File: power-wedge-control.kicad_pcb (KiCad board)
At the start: 2 copper layers, 77.2 x 64.5 mm, 89 parts, among them J1 Conn_01x02, J10 Conn_01x10, J11 Conn_01x08, J12 Conn_01x06, J2 Conn_01x03, J3 Conn_01x02, J4 Conn_01x03, J5 Conn_01x03, J6 Conn_01x06_Female, J7 Conn_01x04_Female, J8 Conn_01x04, J9 MicroSD_Hirose_DM3D-SF, Q1 MMBT3904L, Q2 DMP3099L, Q3 MMBT3904L, Q4 DMP3099L, Q5 MMBT3904L, Q6 MMBT3904L, SW1 SW_SPST, U1 LM1117-5.0, U10 74LVC1G32, U11 74LVC1G32, U2 NC7WZ14P6X, U3 TLV70233DBV, U4 LTV-817S, U5 NC7WZ17P6X, U6 NC7WZ17P6X, U7 LTV-817S, U8 SN74LVC08ADRG3, U9 NC7WZ14P6X

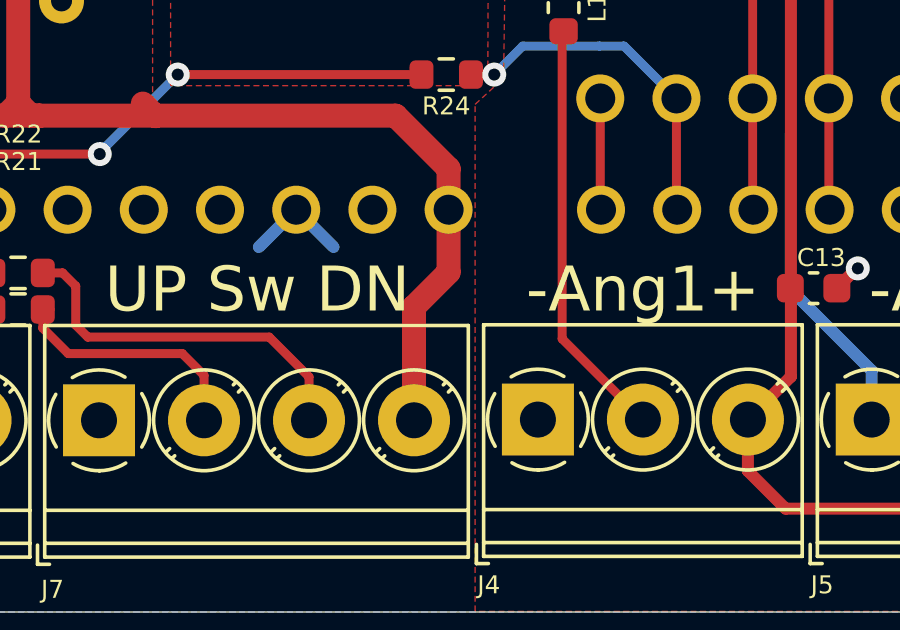
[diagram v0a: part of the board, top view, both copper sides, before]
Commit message: Add 470 Ω resistor to limit current on +12V pin to up/down buttons.
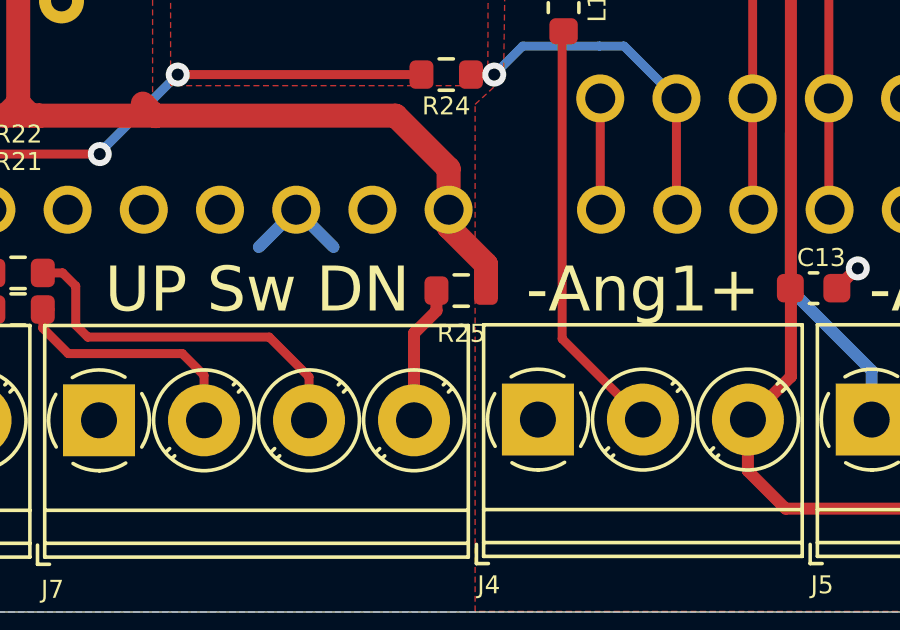
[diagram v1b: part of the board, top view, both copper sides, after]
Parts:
- added R25: 470, Resistor_SMD:R_0603_1608Metric, F.Cu at (168.2, 130.3)
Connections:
- J7 pad 4: +12V -> Net-(J7-Pad4)
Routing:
- net Net-(J7-Pad4): track 0.00 -> 4.63 mm
- net +12V: track 96.6 -> 92.3 mm
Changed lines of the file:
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@@
   (net 80 "Net-(U10-Pad1)")
   (net 81 "Net-(U11-Pad1)")
+  (net 82 "Net-(J7-Pad4)")
   (footprint "TerminalBlock_Phoenix:TerminalBlock_Phoenix_PT-1,5-2-3.5-H_1x02_P3.50mm_Horizontal" (layer "F.Cu")
     (at 126.9088 134.6554)
@@
     )
   )
+  (footprint "Resistor_SMD:R_0603_1608Metric" (layer "F.Cu")
+    (at 168.188 130.331 180)
+    (descr "Resistor SMD 0603 (1608 Metric), square (rectangular) end terminal, IPC_7351 nominal, (Body size source: IPC-SM-782 page 72, https://www.pcb-3d.com/wordpress/wp-content/uploads/ipc-sm-782a_amendment_1_and_2.pdf), generated with kicad-footprint-generator")
+    (tags "resistor")
+    (property "Sheetfile" "power-wedge-control.kicad_sch")
+    (property "Sheetname" "")
+    (attr smd)
+    (fp_text reference "R25" (at 0 -1.43) (layer "F.SilkS")
+      (effects (font (size 0.6 0.6) (thickness 0.15)))
+    )
+    (fp_text value "470" (at 0 1.43) (layer "F.Fab")
+      (effects (font (size 1 1) (thickness 0.15)))
+    )
+    (fp_text user "${REFERENCE}" (at 0 0) (layer "F.Fab")
+      (effects (font (size 0.6 0.6) (thickness 0.06)))
+    )
+    (fp_line (start -0.237258 0.5225) (end 0.237258 0.5225) (layer "F.SilkS") (width 0.12))
+    (fp_line (start -0.237258 -0.5225) (end 0.237258 -0.5225) (layer "F.SilkS") (width 0.12))
+    (fp_line (start -1.48 0.73) (end -1.48 -0.73) (layer "F.CrtYd") (width 0.05))
+    (fp_line (start -1.48 -0.73) (end 1.48 -0.73) (layer "F.CrtYd") (width 0.05))
+    (fp_line (start 1.48 -0.73) (end 1.48 0.73) (layer "F.CrtYd") (width 0.05))
+    (fp_line (start 1.48 0.73) (end -1.48 0.73) (layer "F.CrtYd") (width 0.05))
+    (fp_line (start 0.8 -0.4125) (end 0.8 0.4125) (layer "F.Fab") (width 0.1))
+    (fp_line (start -0.8 0.4125) (end -0.8 -0.4125) (layer "F.Fab") (width 0.1))
+    (fp_line (start -0.8 -0.4125) (end 0.8 -0.4125) (layer "F.Fab") (width 0.1))
+    (fp_line (start 0.8 0.4125) (end -0.8 0.4125) (layer "F.Fab") (width 0.1))
+    (pad "1" smd roundrect (at -0.825 0 180) (size 0.8 0.95) (layers "F.Cu" "F.Paste" "F.Mask") (roundrect_rratio 0.25)
+      (net 4 "+12V") (pintype "passive"))
+    (pad "2" smd roundrect (at 0.825 0 180) (size 0.8 0.95) (layers "F.Cu" "F.Paste" "F.Mask") (roundrect_rratio 0.25)
+      (net 82 "Net-(J7-Pad4)") (pintype "passive"))
+    (model "${KICAD6_3DMODEL_DIR}/Resistor_SMD.3dshapes/R_0603_1608Metric.wrl"
+      (offset (xyz 0 0 0))
+      (scale (xyz 1 1 1))
+      (rotate (xyz 0 0 0))
+    )
+  )
   (footprint "Capacitor_SMD:C_0603_1608Metric" (layer "F.Cu")
     (at 179.9336 130.2512)
@@
       (net 70 "/SW2EXT") (pinfunction "Pin_3") (pintype "passive"))
     (pad "4" thru_hole circle locked (at 10.5 0) (size 2.4 2.4) (drill 1.2) (layers *.Cu *.Mask)
-      (net 4 "+12V") (pinfunction "Pin_4") (pintype "passive"))
+      (net 82 "Net-(J7-Pad4)") (pinfunction "Pin_4") (pintype "passive"))
     (model "${KICAD6_3DMODEL_DIR}/TerminalBlock_Phoenix.3dshapes/TerminalBlock_Phoenix_PT-1,5-4-3.5-H_1x04_P3.50mm_Horizontal.wrl"
       (offset (xyz 0 0 0))
@@
   (segment (start 115.8224 124.8664) (end 115.8224 123.4668) (width 0.8) (layer "F.Cu") (net 3))
   (segment (start 153 124.5) (end 154.138 124.5) (width 0.8) (layer "F.Cu") (net 4))
+  (segment (start 169.013 130.331) (end 169.013 129.456) (width 0.8) (layer "F.Cu") (net 4))
   (segment (start 154.9562 115.9502) (end 155.6562 115.2502) (width 0.8) (layer "F.Cu") (net 4))
   (segment (start 119.198 120.4346) (end 119.198 119.0244) (width 0.8) (layer "F.Cu") (net 4))
@@
   (segment (start 154.138 124.5) (end 166 124.5) (width 0.8) (layer "F.Cu") (net 4))
   (segment (start 153.421 115.9502) (end 153.421 124.079) (width 0.8) (layer "F.Cu") (net 4))
-  (segment (start 167.767 129.7178) (end 166.6136 130.8712) (width 0.8) (layer "F.Cu") (net 4))
   (segment (start 127.741518 124.499118) (end 126.9088 125.331836) (width 0.8) (layer "F.Cu") (net 4))
   (segment (start 154.138 124.5) (end 153.842 124.5) (width 0.8) (layer "F.Cu") (net 4))
-  (segment (start 166.6136 130.8712) (end 166.6136 134.6554) (width 0.8) (layer "F.Cu") (net 4))
   (segment (start 126.119 120.4346) (end 126.6656 119.888) (width 0.8) (layer "F.Cu") (net 4))
   (segment (start 132.650482 124.499118) (end 132.6878 124.4618) (width 0.8) (layer "F.Cu") (net 4))
@@
   (segment (start 122.566 119.0092) (end 122.6524 118.9228) (width 0.8) (layer "F.Cu") (net 4))
   (segment (start 126.9088 125.331836) (end 126.9088 134.6554) (width 0.8) (layer "F.Cu") (net 4))
-  (segment (start 167.767 127.635) (end 167.767 129.7178) (width 0.8) (layer "F.Cu") (net 4))
   (segment (start 147.8788 124.5) (end 153 124.5) (width 0.8) (layer "F.Cu") (net 4))
   (segment (start 126.056 120.4346) (end 126.119 120.4346) (width 0.8) (layer "F.Cu") (net 4))
@@
   (segment (start 155.6562 115.2502) (end 155.6562 116.3832) (width 0.8) (layer "F.Cu") (net 4))
   (segment (start 116.5056 118.9228) (end 119.0964 118.9228) (width 0.8) (layer "F.Cu") (net 4))
+  (segment (start 169.013 129.456) (end 167.767 128.21) (width 0.8) (layer "F.Cu") (net 4))
   (segment (start 115.708 120.7562) (end 115.708 119.7204) (width 0.8) (layer "F.Cu") (net 4))
   (segment (start 125.7004 118.9228) (end 126.6656 119.888) (width 0.8) (layer "F.Cu") (net 4))
   (segment (start 153.842 124.5) (end 153.421 124.079) (width 0.8) (layer "F.Cu") (net 4))
   (segment (start 153.421 124.079) (end 153 124.5) (width 0.8) (layer "F.Cu") (net 4))
+  (segment (start 167.767 128.21) (end 167.767 127.635) (width 0.8) (layer "F.Cu") (net 4))
   (segment (start 142.388 124.481) (end 132.650482 124.499118) (width 0.8) (layer "F.Cu") (net 4))
   (via (at 147.8788 124.5) (size 1.6) (drill 0.8) (layers "F.Cu" "B.Cu") (net 4))
@@
   (segment (start 128.239519 94.874519) (end 128.89 95.525) (width 0.3) (layer "F.Cu") (net 81))
   (segment (start 128.89 95.525) (end 128.89 97.7) (width 0.3) (layer "F.Cu") (net 81))
+  (segment (start 167.363 130.331) (end 167.363 131.006) (width 0.4) (layer "F.Cu") (net 82))
+  (segment (start 167.363 131.006) (end 166.6136 131.7554) (width 0.4) (layer "F.Cu") (net 82))
+  (segment (start 166.6136 131.7554) (end 166.6136 134.6554) (width 0.4) (layer "F.Cu") (net 82))
   (zone (net 0) (net_name "") (layer "F.Cu") (hatch edge 0.508)
     (connect_pads (clearance 0))
